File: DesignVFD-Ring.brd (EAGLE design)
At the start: 160 x 100 mm, 34 parts, among them IC1 LMR64010XMF/NOPB, IC2 LM340S-05, U1 MAX6920AWP+, U2 LM1084IS-5.0, U3 TPS76325DBVT

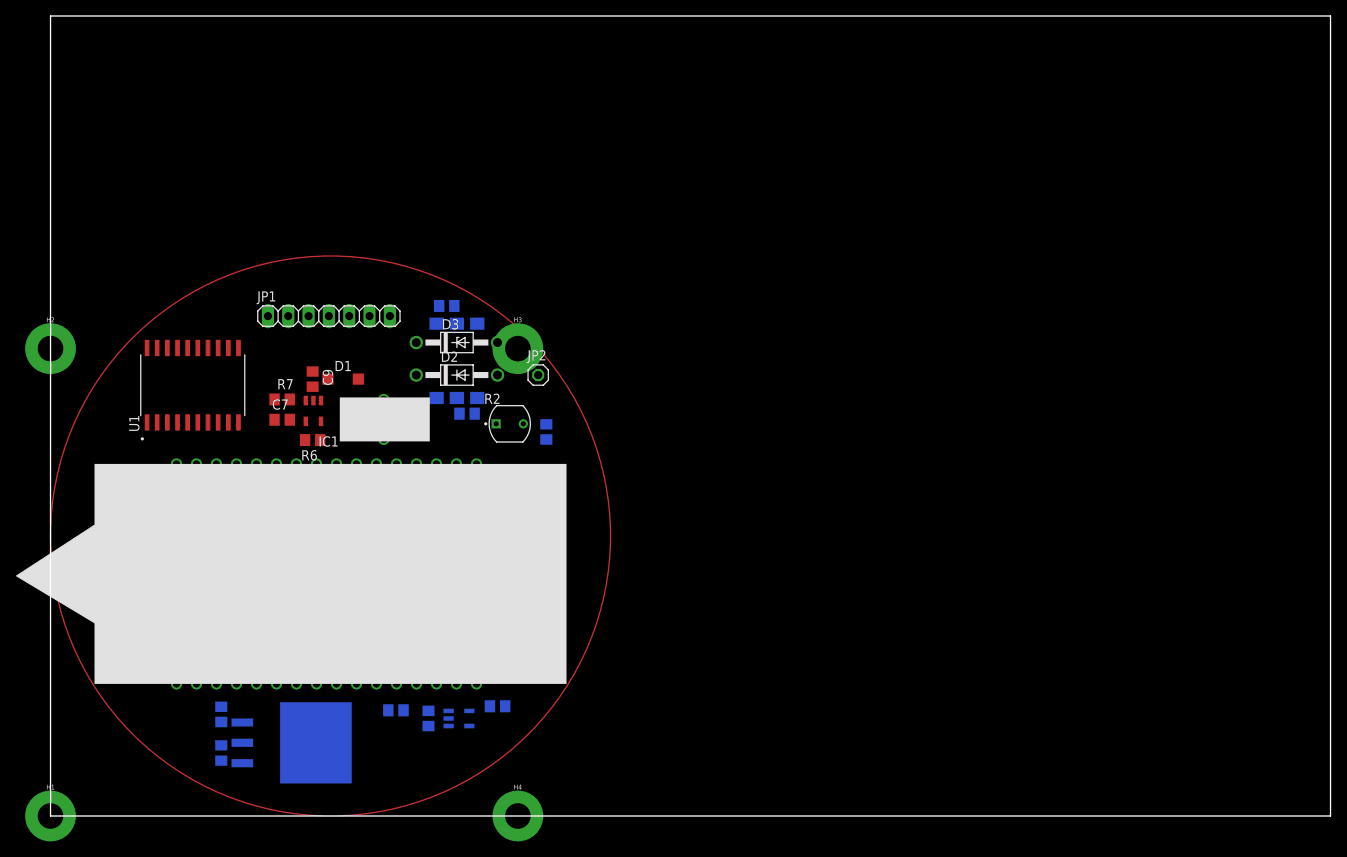
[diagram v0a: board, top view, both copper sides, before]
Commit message: about to repin IVL
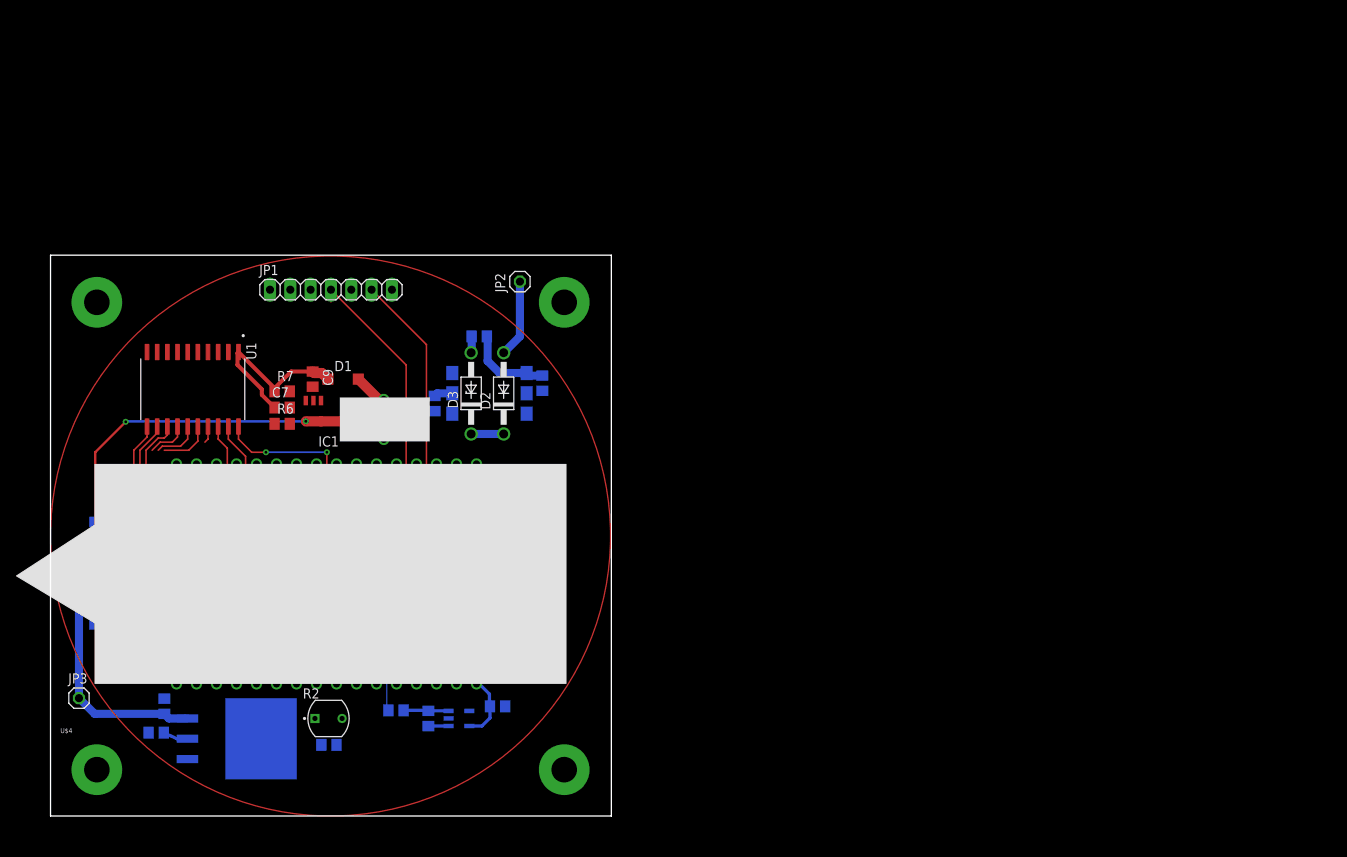
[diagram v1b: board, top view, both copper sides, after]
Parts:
- removed H1, H2, H3, H4: STANDOFF_ELECTRICAL, SparkFun-Hardware:STANDOFF-ELECTRICAL
- added JP3: (no value), pinhead:1X01
- added U$4: LUMINI3, FormE:STANDOFF-ELECTRICAL
- moved R3 47.6 mm to (34.8, 8.89), turned to 0 degrees
- moved R2 43.2 mm to (34.7, 12.2)
- moved C2 12.3 mm to (48.0, 51.6), turned to 270 degrees
- moved JP2 11.9 mm to (58.7, 66.8), turned to 90 degrees
- moved C1 10.1 mm to (61.5, 54.1), turned to 270 degrees
- moved C4 8.52 mm to (13.2, 10.4), turned to 0 degrees
- moved C3 7.18 mm to (14.2, 13.7)
- moved U2 6.88 mm to (26.2, 9.65)
- moved D3 6.59 mm to (52.6, 52.8), turned to 90 degrees
- moved C8 6.55 mm to (5.59, 35.8), turned to 90 degrees
- moved D2 6.27 mm to (56.6, 52.8), turned to 90 degrees
- moved IC2 6.15 mm to (11.4, 30.2)
- moved C6 6.15 mm to (5.59, 24.9), turned to 270 degrees
- moved OK1 5.75 mm to (54.9, 52.8), turned to 270 degrees
- moved R1 5.01 mm to (53.6, 59.9), turned to 180 degrees
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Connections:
- net +15V: now also JP3.1
- net GND: now also U$4.P1, U$4.P2, U$4.P3, U$4.P4; no longer H1.P1, H2.P1, H3.P1, H4.P1
- net T_CS2: now also U$3.3; no longer U$3.5
- net T_MOSI2: now also U$3.5; no longer U$3.3
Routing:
- net T_SCK: track 0.00 -> 59.1 mm, vias 0 -> 1
- net +12V: track 0.00 -> 51.3 mm, vias 0 -> 3
- net N$12: track 0.00 -> 48.5 mm, vias 0 -> 1
- net T_MOSI: track 0.00 -> 45.1 mm, vias 0 -> 1
- net T_CS2: track 0.00 -> 36.7 mm, vias 0 -> 1
- net +3V3: track 0.00 -> 34.7 mm, vias 0 -> 3
- net T_SCK2: track 0.00 -> 33.3 mm, vias 0 -> 1
- net +15V: track 0.00 -> 29.8 mm
- net T_MOSI2: track 0.00 -> 28.0 mm, vias 0 -> 1
- net +24V: track 0.00 -> 23.6 mm
- net N$4: track 0.00 -> 10.7 mm
- net IGN_INPUT: track 0.00 -> 9.73 mm
- net V+: track 0.00 -> 8.15 mm
- net T_HEATER_CTL: track 0.00 -> 7.86 mm
- net N$5: track 0.00 -> 7.25 mm
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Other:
- board size 160 x 100 mm -> 70.1 x 70.1 mm
